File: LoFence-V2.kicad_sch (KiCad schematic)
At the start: 55 parts, among them J1 Fence+, J2 Fence-, Q1 LBSS84LT1G, Q2 MMBT3904, SW1 RESET, SW2 ACTIVATE, U1 TPS63051RMW, U2 TLV9062, U3 ATmega328PB-AU, U4 LA66, Y1 32768 Hz

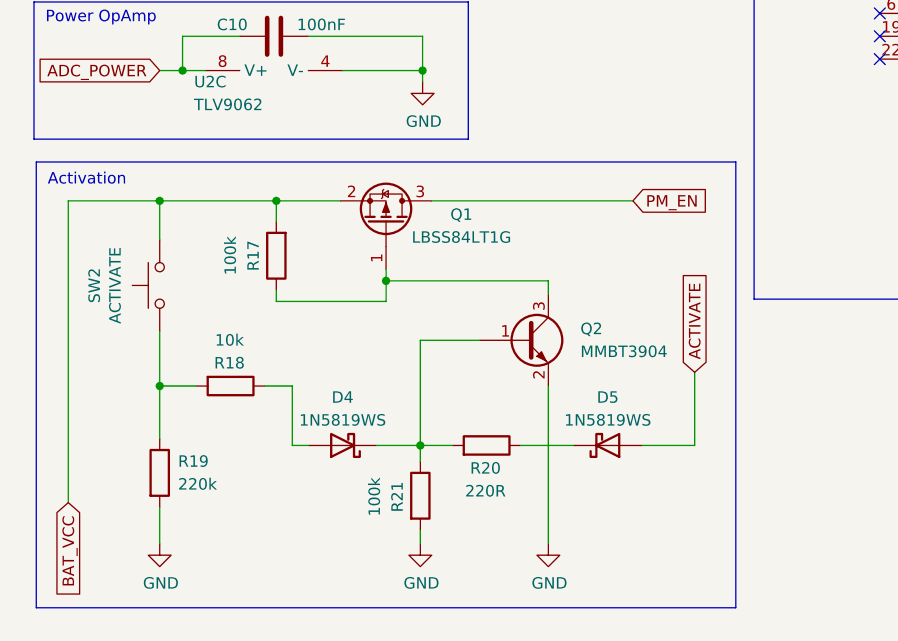
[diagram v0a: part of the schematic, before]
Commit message: switch Q2 to a N-MOSFET and simplify activation circuit
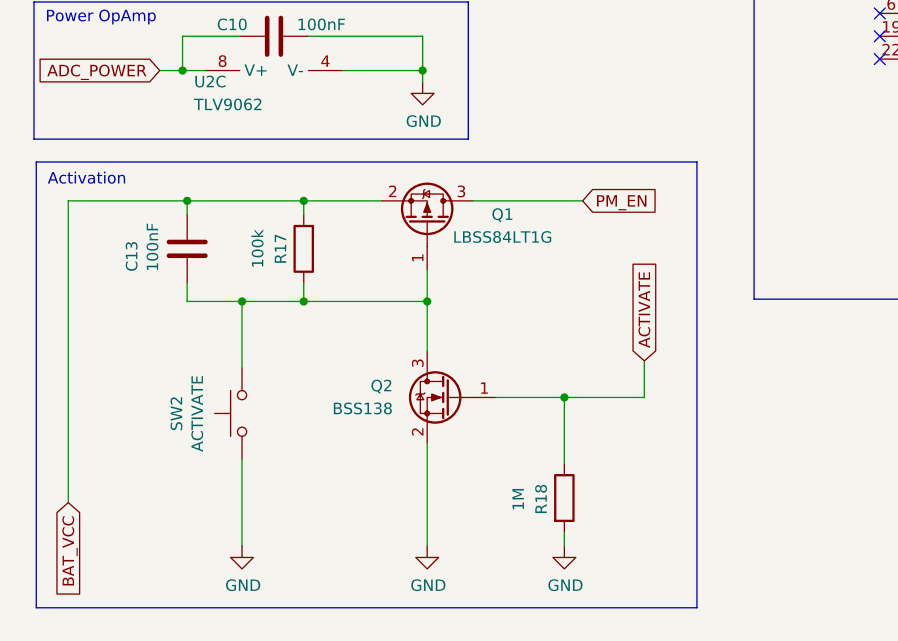
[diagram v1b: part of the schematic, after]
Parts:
- removed D4, D5: 1N5819WS, Diode_SMD:D_SOD-323, symbol Diode:1N5819WS
- removed Q2: MMBT3904, Package_TO_SOT_SMD:SOT-23, symbol Transistor_BJT:MMBT3904
- removed R18: 10k, Resistor_SMD:R_0603_1608Metric_Pad0.98x0.95mm_HandSolder, symbol Device:R
- removed R19: 220k, Resistor_SMD:R_0603_1608Metric_Pad0.98x0.95mm_HandSolder, symbol Device:R
- removed R20: 220R, Resistor_SMD:R_0603_1608Metric_Pad0.98x0.95mm_HandSolder, symbol Device:R
- added C13: 100nF, Capacitor_SMD:C_0805_2012Metric_Pad1.18x1.45mm_HandSolder, symbol Device:C
- added Q2: BSS138, Package_TO_SOT_SMD:SOT-23, symbol Transistor_FET:BSS138
- R18: renamed from R21; value 100k -> 1M
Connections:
- net ACTIVATE: now also R18.1, Q2.1 (G)
- net BAT_VCC: now also C13.1; no longer SW2.1
- net GND: now also SW2.2, Q2.2 (S)
- net at Q1.1 (G), R17.1: now also SW2.1, C13.2, Q2.3 (D)
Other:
- moved on the sheet: Q1, R17, R18, SW2
